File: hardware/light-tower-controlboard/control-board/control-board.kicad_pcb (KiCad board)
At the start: 2 copper layers, 7 parts, among them J1 DE9, J2 VIN, J5 Conn_01x02

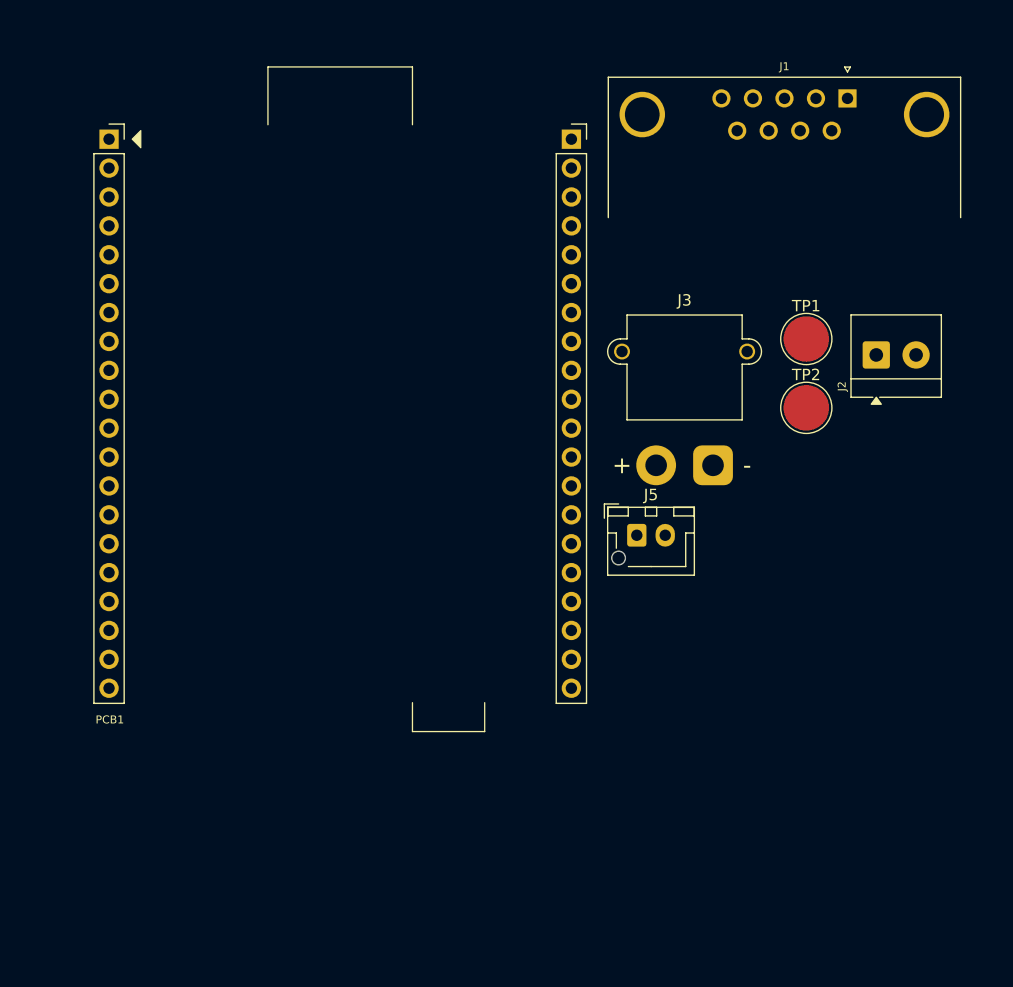
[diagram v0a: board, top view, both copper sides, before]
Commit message: finalised design and ready for manufacture
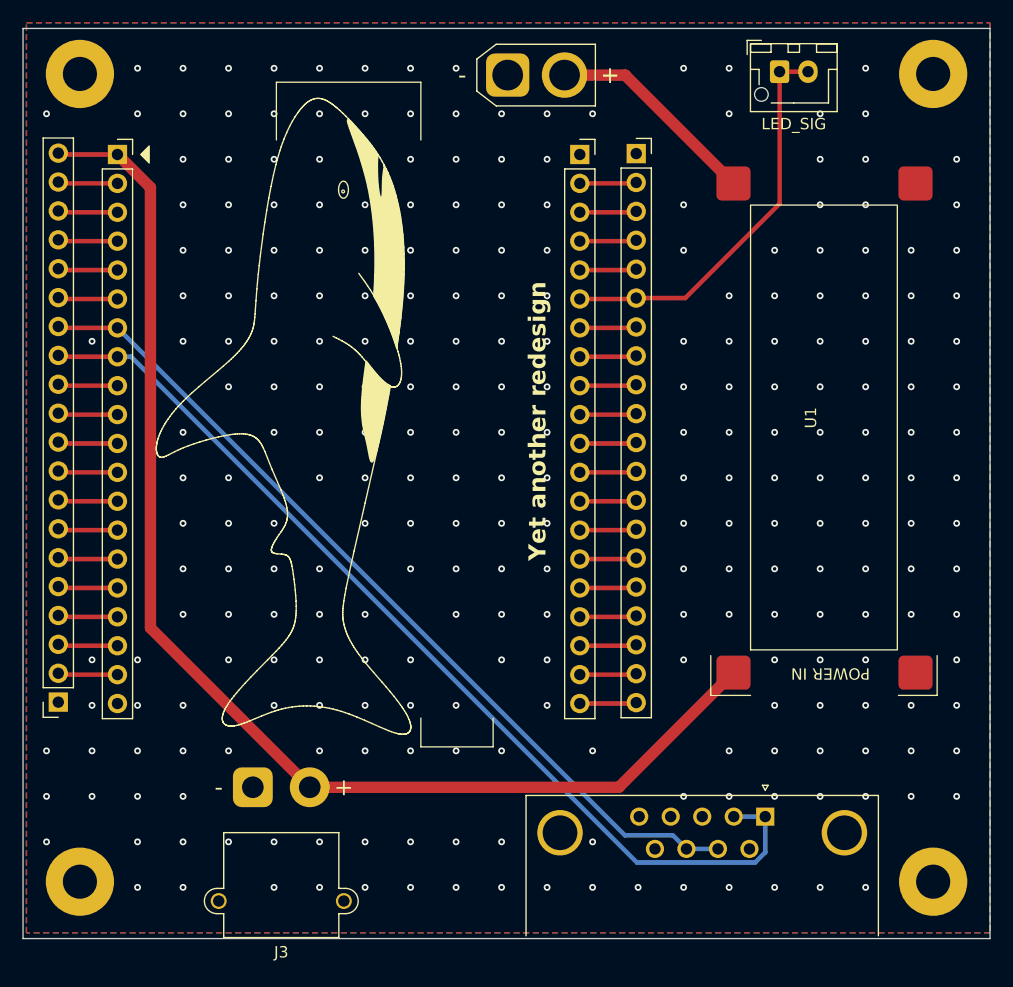
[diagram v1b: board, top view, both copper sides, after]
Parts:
- removed TP1: GND, TestPoint:TestPoint_Pad_D4.0mm
- removed TP2: LED_VOUT, TestPoint:TestPoint_Pad_D4.0mm
- added H1: MountingHole_Pad, MountingHole:MountingHole_3mm_Pad, F.Cu at (135.0, 44.0)
- added H2: MountingHole_Pad, MountingHole:MountingHole_3mm_Pad, F.Cu at (135.0, 115.0)
- added H3: MountingHole_Pad, MountingHole:MountingHole_3mm_Pad, F.Cu at (60.0, 44.0)
- added H4: MountingHole_Pad, MountingHole:MountingHole_3mm_Pad, F.Cu at (60.0, 115.0)
- added J4: ~, Connector_AMASS:AMASS_XT30U-F_1x02_P5.0mm_Vertical, F.Cu at (97.6, 44.1)
- added J6: Conn_01x20, Connector_PinSocket_2.54mm:PinSocket_1x20_P2.54mm_Vertical, F.Cu at (108.9, 51.0)
- added REF**: Smolhaj_Scale_0.1, Symbol:Smolhaj_Scale_0.1, F.Cu at (81.0, 46.1)
- added U1: ~, Library:LM2596_reg_module, F.Cu at (112.5, 96.6)
- J2: value VIN -> Conn_01x20; footprint Library:TerminalBlock_4Ucon_1x02_P3.50mm_Horizontal -> Connector_PinSocket_2.54mm:PinSocket_1x20_P2.54mm_Vertical
- J5: value Conn_01x02 -> LED_SIG
- moved J2 78.1 mm to (58.1, 99.2), turned to 180 degrees
- moved J1 63.5 mm to (120.2, 109.3)
- moved J3 49.4 mm to (75.2, 106.7), turned to 180 degrees
- moved J5 42.6 mm to (121.5, 43.8)
- moved PCB1 1.54 mm to (83.6, 75.2)
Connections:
- net Net-(J5-Pin_1) renamed /LED_SIG
- J1 pad 1: Net-(PCB1-CAN_L) -> /CAN_L
- J1 pad 2: Net-(PCB1-CAN_L) -> /CAN_L
- J1 pad 7: Net-(PCB1-CAN_H) -> /CAN_H
- J1 pad 8: Net-(PCB1-CAN_H) -> /CAN_H
- J2 pad 2: VCC -> Net-(J2-Pin_2)
- PCB1 pad 1: +5V -> VCC
- PCB1 pad 10: unconnected-(PCB1-A2-Pad10) -> Net-(J2-Pin_11)
- PCB1 pad 11: unconnected-(PCB1-A3-Pad11) -> Net-(J2-Pin_10)
- PCB1 pad 12: unconnected-(PCB1-A4-Pad12) -> Net-(J2-Pin_9)
- PCB1 pad 13: unconnected-(PCB1-A5-Pad13) -> Net-(J2-Pin_8)
- PCB1 pad 14: unconnected-(PCB1-A6-Pad14) -> Net-(J2-Pin_7)
- PCB1 pad 15: unconnected-(PCB1-A7-Pad15) -> Net-(J2-Pin_6)
- PCB1 pad 16: unconnected-(PCB1-A8-Pad16) -> Net-(J2-Pin_5)
- PCB1 pad 17: unconnected-(PCB1-A9-Pad17) -> Net-(J2-Pin_4)
- PCB1 pad 18: unconnected-(PCB1-A10-Pad18) -> Net-(J2-Pin_3)
- PCB1 pad 19: unconnected-(PCB1-IO12-Pad19) -> Net-(J2-Pin_2)
- PCB1 pad 2: unconnected-(PCB1-LED_DOUT-Pad2) -> Net-(J2-Pin_19)
- PCB1 pad 21: unconnected-(PCB1-3V3-Pad21) -> Net-(J6-Pin_20)
- PCB1 pad 22: unconnected-(PCB1-IO13-Pad22) -> Net-(J6-Pin_19)
- PCB1 pad 23: unconnected-(PCB1-IO14-Pad23) -> Net-(J6-Pin_18)
- PCB1 pad 24: unconnected-(PCB1-IO21-Pad24) -> Net-(J6-Pin_17)
- PCB1 pad 25: unconnected-(PCB1-IO47-Pad25) -> Net-(J6-Pin_16)
- PCB1 pad 26: unconnected-(PCB1-IO48-Pad26) -> Net-(J6-Pin_15)
- PCB1 pad 27: unconnected-(PCB1-IO45-Pad27) -> Net-(J6-Pin_14)
- PCB1 pad 28: unconnected-(PCB1-IO37-Pad28) -> Net-(J6-Pin_13)
- PCB1 pad 29: unconnected-(PCB1-IO38-Pad29) -> Net-(J6-Pin_12)
- PCB1 pad 3: unconnected-(PCB1-UART0_TX-Pad3) -> Net-(J2-Pin_18)
- PCB1 pad 30: unconnected-(PCB1-IO39-Pad30) -> Net-(J6-Pin_11)
- PCB1 pad 31: unconnected-(PCB1-IO40-Pad31) -> Net-(J6-Pin_10)
- PCB1 pad 32: unconnected-(PCB1-IO41-Pad32) -> Net-(J6-Pin_9)
- PCB1 pad 33: unconnected-(PCB1-IO42-Pad33) -> Net-(J6-Pin_8)
- PCB1 pad 34: unconnected-(PCB1-IO16-Pad34) -> Net-(J6-Pin_7)
- PCB1 pad 36: unconnected-(PCB1-CAN_RX-Pad36) -> Net-(J6-Pin_5)
- PCB1 pad 37: unconnected-(PCB1-CAN_TX-Pad37) -> Net-(J6-Pin_4)
- PCB1 pad 38: unconnected-(PCB1-I2C_SDA-Pad38) -> Net-(J6-Pin_3)
- PCB1 pad 39: unconnected-(PCB1-I2C_SCK-Pad39) -> Net-(J6-Pin_2)
- PCB1 pad 4: unconnected-(PCB1-UART0_RX-Pad4) -> Net-(J2-Pin_17)
- PCB1 pad 5: unconnected-(PCB1-UART1_TX-Pad5) -> Net-(J2-Pin_16)
- PCB1 pad 6: unconnected-(PCB1-UART1_RX-Pad6) -> Net-(J2-Pin_15)
- PCB1 pad 7: Net-(PCB1-CAN_H) -> /CAN_H
- PCB1 pad 8: Net-(PCB1-CAN_L) -> /CAN_L
- PCB1 pad 9: unconnected-(PCB1-A1-Pad9) -> Net-(J2-Pin_12)
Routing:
- net VCC: track 0.00 -> 109.3 mm
- net /CAN_L: track 0.00 -> 86.9 mm
- net /CAN_H: track 0.00 -> 77.0 mm
- net /LED_SIG: track 0.00 -> 35.1 mm
- net VBUS: track 0.00 -> 18.8 mm
- net Net-(J2-Pin_8): track 0.00 -> 5.25 mm
- net Net-(J2-Pin_6): track 0.00 -> 5.25 mm
- net Net-(J2-Pin_5): track 0.00 -> 5.25 mm
- net Net-(J2-Pin_4): track 0.00 -> 5.25 mm
- net Net-(J2-Pin_3): track 0.00 -> 5.25 mm
- net Net-(J2-Pin_17): track 0.00 -> 5.25 mm
- net Net-(J2-Pin_16): track 0.00 -> 5.25 mm
- net Net-(J2-Pin_15): track 0.00 -> 5.25 mm
- net Net-(J2-Pin_12): track 0.00 -> 5.25 mm
- net Net-(J2-Pin_11): track 0.00 -> 5.25 mm
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- added copper zone on B.Cu, net GND
- added copper zone on F.Cu, net GND
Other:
- board outline added: 85 x 80 mm
- board text added: "Designed by MRB"
- board text added: "Yet another redesign"
